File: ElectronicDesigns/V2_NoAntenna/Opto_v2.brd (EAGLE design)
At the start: 27.6 x 14 mm, 7 parts

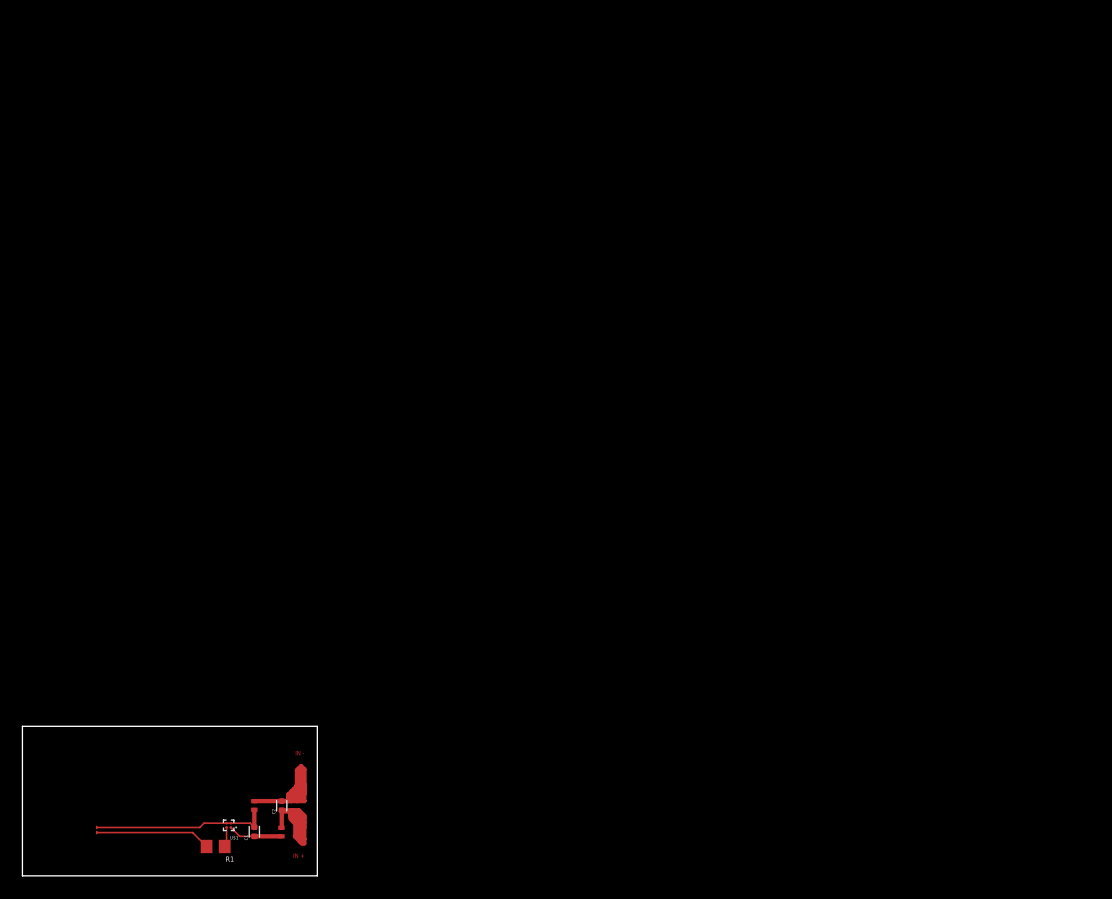
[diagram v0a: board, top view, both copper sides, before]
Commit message: Update gerbers
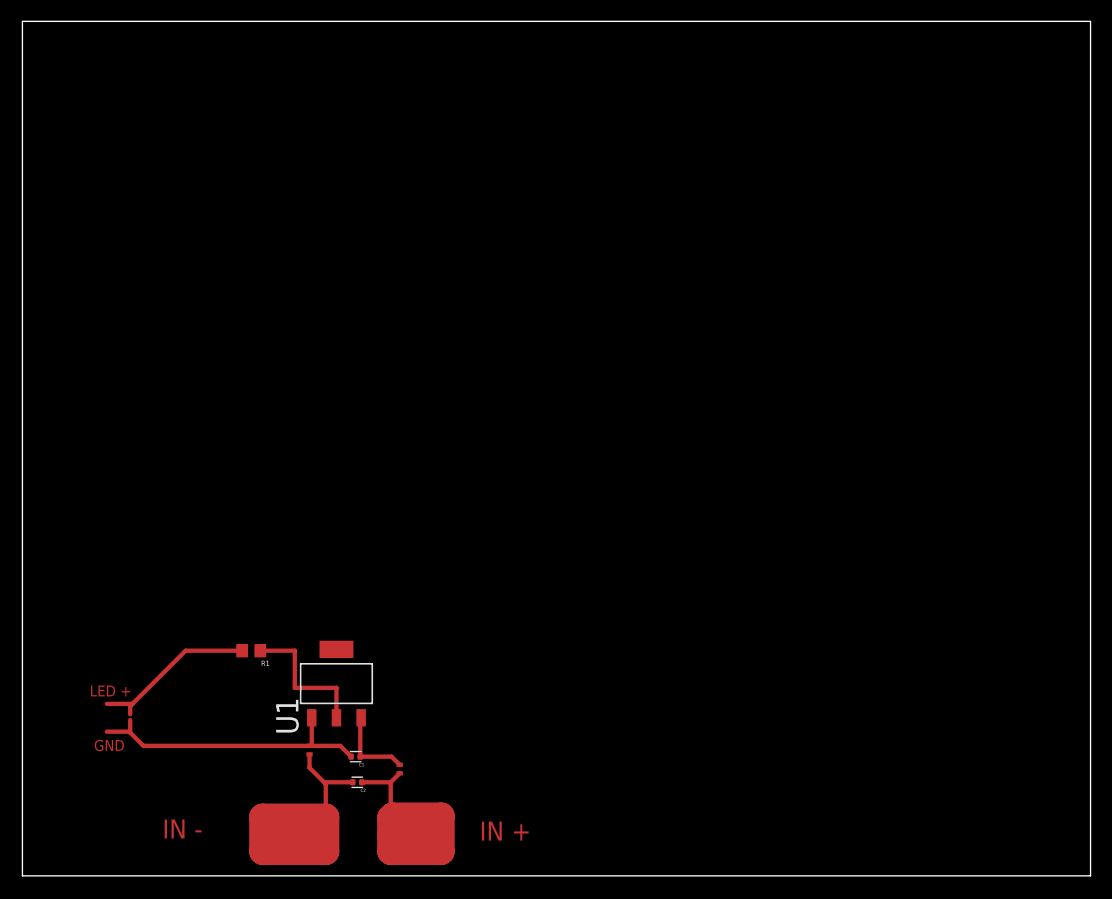
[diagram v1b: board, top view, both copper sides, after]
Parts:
- removed U$1: BGA4C4, LOD_BGA4C40P2X2_84X84X60N:BGA4C40P2X2_84X84X60N
- added U1: TLV1117-18IDCYG3, TLV1117-18IDCYG3:SOT230P700X180-4N
- moved R1 18.6 mm to (21.4, 21.1)
- moved U$2 12.5 mm to (35.3, 10.0), turned to 90 degrees
- moved C1 11.8 mm to (31.2, 11.2), turned to 180 degrees
- moved U$4 11.0 mm to (10.1, 14.8), turned to 270 degrees
- moved C2 7.40 mm to (31.4, 8.76), turned to 180 degrees
- moved U$3 7.32 mm to (26.9, 11.8), turned to 270 degrees
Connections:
- net GND: now also U1.1; no longer U$1.B1, U$1.B2
- net N$1: now also U1.2; no longer U$1.A2
- net N$4: now also U1.3; no longer U$1.A1
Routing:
- net N$1: track 1.85 -> 13.4 mm
- net GND: track 16.7 -> 27.6 mm
- net N$2: track 10.8 -> 15.8 mm
- net IN+: track 22.4 -> 26.5 mm
- net IN-: track 28.2 -> 32.2 mm
- net N$4: track 5.08 -> 7.68 mm
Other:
- board size 27.6 x 14 mm -> 100 x 80 mm
- board text added: "GND"
- board text added: "LED +"

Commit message: Updated gerbers
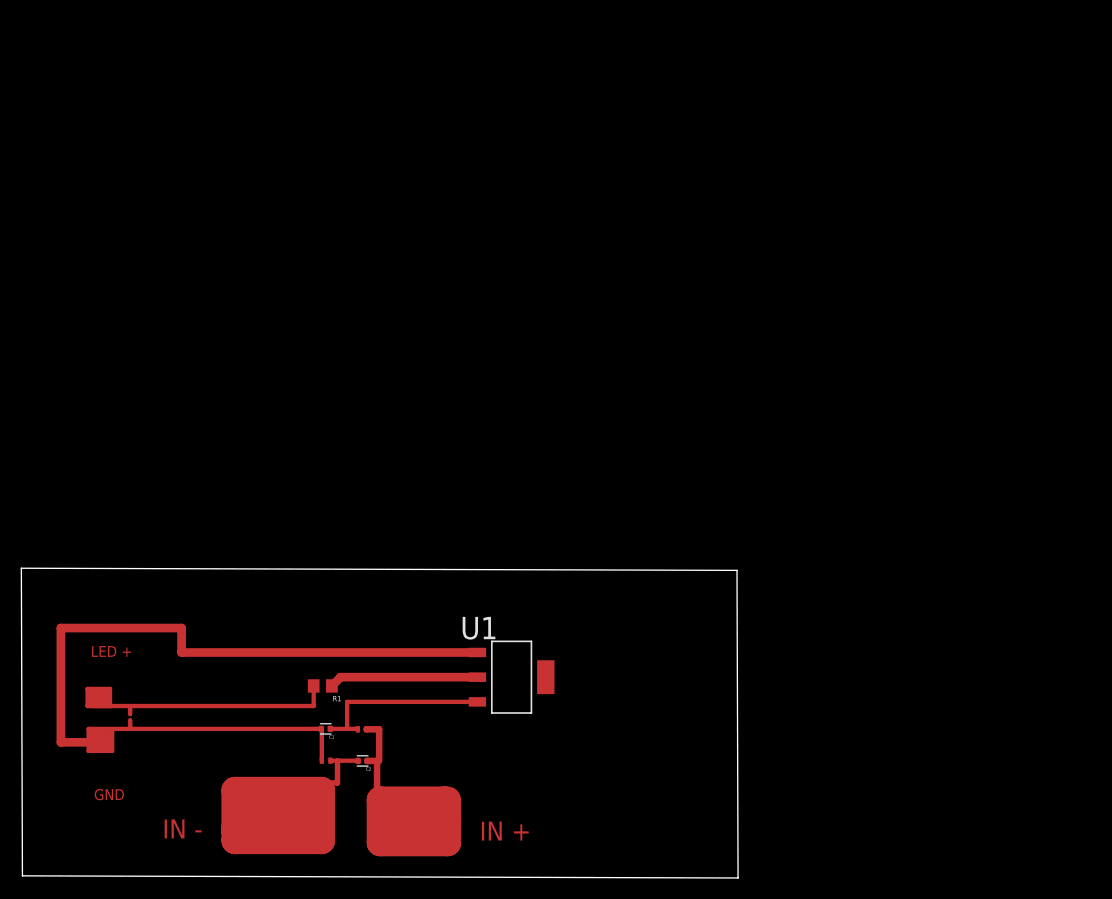
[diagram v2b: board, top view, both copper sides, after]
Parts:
- moved U1 16.4 mm to (45.8, 18.6), turned to 0 degrees
- moved R1 7.47 mm to (28.1, 17.8)
- moved U$2 5.12 mm to (31.8, 13.7), turned to 180 degrees
- moved C1 3.82 mm to (28.4, 13.8)
- moved C2 2.06 mm to (31.9, 10.8)
- moved U$3 1.84 mm to (28.4, 10.8), turned to 0 degrees
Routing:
- net GND: track 27.6 -> 98.0 mm
- net IN-: track 32.2 -> 55.2 mm
- net N$2: track 15.8 -> 38.5 mm
- net IN+: track 26.5 -> 45.7 mm
- net N$4: track 7.68 -> 17.3 mm
- net N$1: track 13.4 -> 14.0 mm
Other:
- board size 100 x 80 mm -> 67.1 x 29 mm
